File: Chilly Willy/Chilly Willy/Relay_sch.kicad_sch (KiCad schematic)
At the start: 4 parts, among them K1 AGQ200A4H, Q2 2N7000

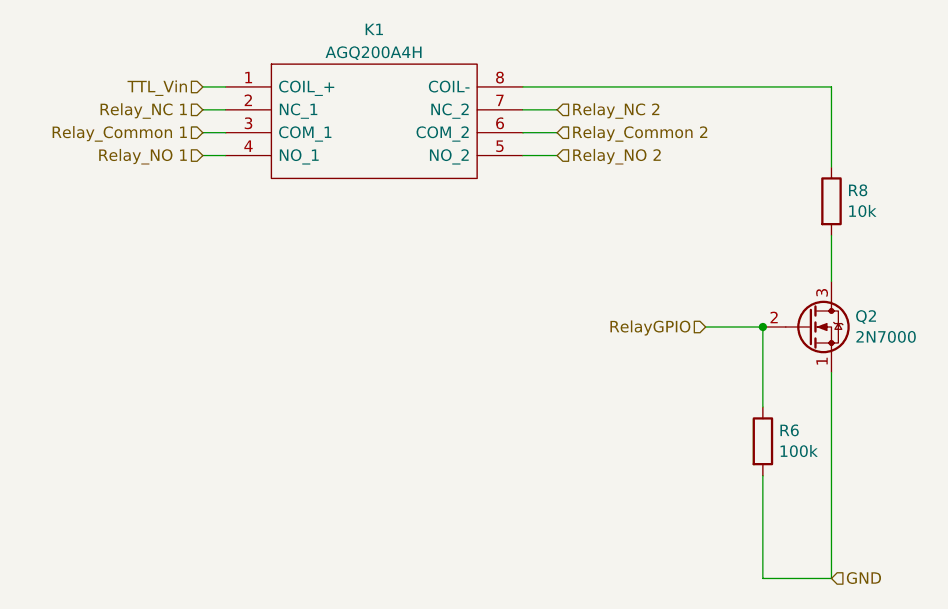
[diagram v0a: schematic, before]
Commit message: ..
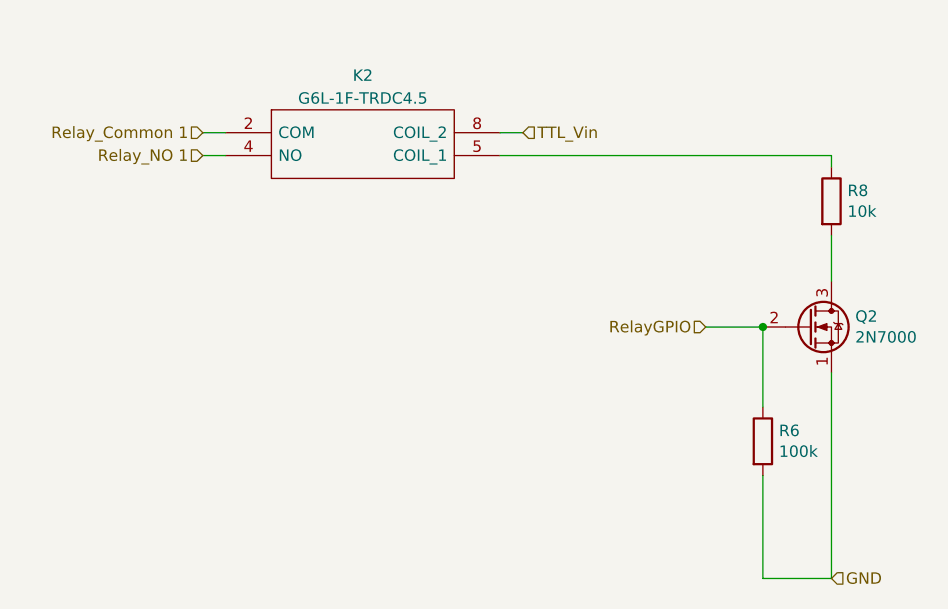
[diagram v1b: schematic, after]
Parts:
- removed K1: AGQ200A4H, AGQ200A12, symbol SamacSys_Parts:AGQ200A4H
- added K2: G6L-1F-TRDC4.5, G6L1FTRDC45, symbol SamacSys_Parts:G6L-1F-TRDC4.5
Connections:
- net Relay_Common 1: now also K2.2 (COM)
- net Relay_NO 1: now also K2.4 (NO)
- net TTL_Vin: now also K2.8 (COIL_2)
- net at R8.1: now also K2.5 (COIL_1)
